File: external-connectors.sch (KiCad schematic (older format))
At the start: 7 parts, among them J1 Barrel_Jack +5V, J2 Barrel_Jack +12V, J3 Conn_02x10_Odd_Even, J4 Conn_02x08_Odd_Even, J5 Conn_02x08_Odd_Even

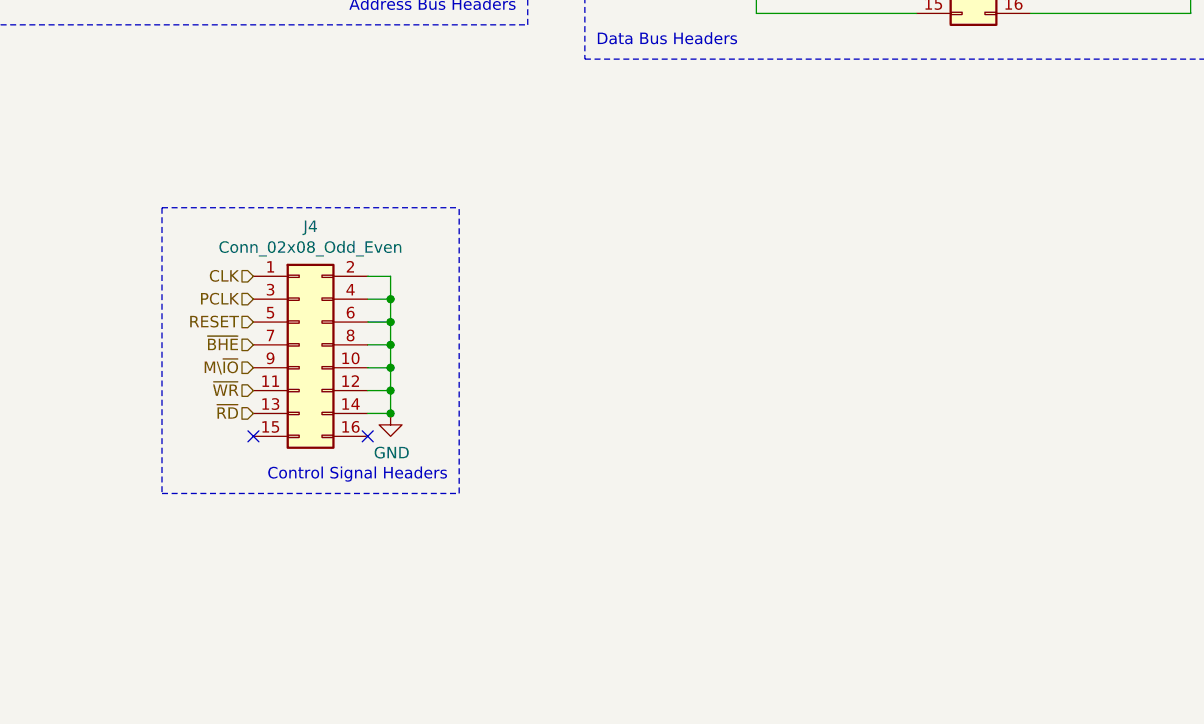
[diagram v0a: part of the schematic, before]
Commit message: assign footprints and edits
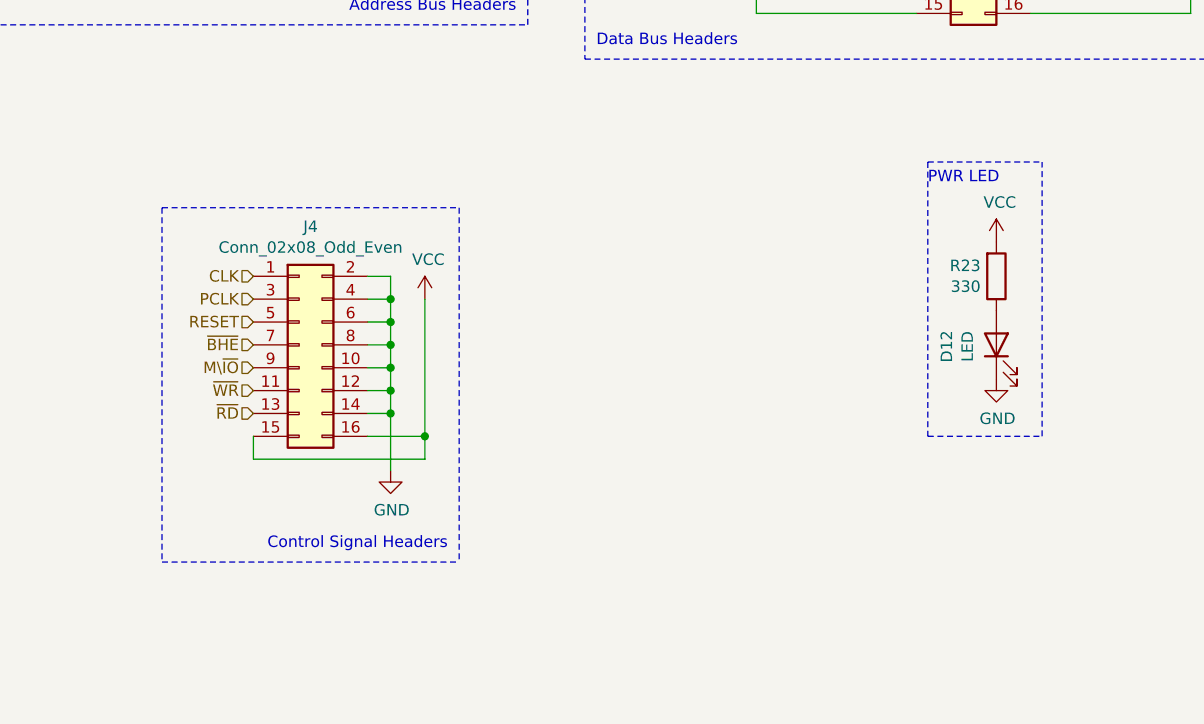
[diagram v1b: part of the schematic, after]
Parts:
- added D12: LED, LED_THT:LED_D5.0mm, symbol Device:LED
- added R23: 330, Resistor_THT:R_Axial_DIN0207_L6.3mm_D2.5mm_P10.16mm_Horizontal, symbol Device:R
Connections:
- net GND: now also D12.1 (K)
- net VCC: now also J4.15 (Pin_15), J4.16 (Pin_16), R23.2
- new net: D12.2 (A), R23.1
- no-connect marks 2 -> 0
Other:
- note added: "PWR LED"
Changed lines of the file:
@@
 $EndComp
 Wire Notes Line
-	3700 4450 3700 5700
-Wire Notes Line
-	3700 5700 5000 5700
-Wire Notes Line
-	5000 5700 5000 4450
+	3700 6000 5000 6000
 Wire Notes Line
 	3700 4450 5000 4450
-Text Notes 4950 5650 2    50   ~ 0
+Text Notes 4950 5950 2    50   ~ 0
 Control Signal Headers
 Text HLabel 4100 5150 0    50   Input ~ 0
@@
 Text HLabel 4100 5350 0    50   Input ~ 0
 ~RD
-NoConn ~ 4100 5450
-NoConn ~ 4600 5450
 Wire Wire Line
 	4600 4750 4700 4750
@@
 L power:GND #PWR0105
 U 1 1 62100CCC
-P 4700 5350
-F 0 "#PWR0105" H 4700 5100 50  0001 C CNN
-F 1 "GND" H 4705 5177 50  0000 C CNN
-F 2 "" H 4700 5350 50  0001 C CNN
-F 3 "" H 4700 5350 50  0001 C CNN
-	1    4700 5350
+P 4700 5600
+F 0 "#PWR0105" H 4700 5350 50  0001 C CNN
+F 1 "GND" H 4705 5427 50  0000 C CNN
+F 2 "" H 4700 5600 50  0001 C CNN
+F 3 "" H 4700 5600 50  0001 C CNN
+	1    4700 5600
 	1    0    0    -1
 $EndComp
@@
 	4700 5250 4700 5350
 Connection ~ 4700 5250
-Connection ~ 4700 5350
 $Comp
 L power:PWR_FLAG #FLG0101
@@
 	2450 5500 1850 5500
 Connection ~ 1850 5500
+Text Notes 7050 4350 0    50   ~ 0
+PWR LED
+$Comp
+L power:VCC #PWR02
+U 1 1 61BA534A
+P 7350 4600
+F 0 "#PWR02" H 7350 4450 50  0001 C CNN
+F 1 "VCC" H 7365 4773 50  0000 C CNN
+F 2 "" H 7350 4600 50  0001 C CNN
+F 3 "" H 7350 4600 50  0001 C CNN
+	1    7350 4600
+	1    0    0    -1
+$EndComp
+$Comp
+L power:GND #PWR03
+U 1 1 61BA5A77
+P 7350 5200
+F 0 "#PWR03" H 7350 4950 50  0001 C CNN
+F 1 "GND" H 7355 5027 50  0000 C CNN
+F 2 "" H 7350 5200 50  0001 C CNN
+F 3 "" H 7350 5200 50  0001 C CNN
+	1    7350 5200
+	1    0    0    -1
+$EndComp
+Wire Wire Line
+	4100 5450 4100 5550
+Wire Wire Line
+	4100 5550 4850 5550
+Wire Wire Line
+	4850 5550 4850 5450
+Wire Wire Line
+	4700 5600 4700 5350
+Connection ~ 4700 5350
+$Comp
+L power:VCC #PWR01
+U 1 1 61BBFA03
+P 4850 4850
+F 0 "#PWR01" H 4850 4700 50  0001 C CNN
+F 1 "VCC" H 4865 5023 50  0000 C CNN
+F 2 "" H 4850 4850 50  0001 C CNN
+F 3 "" H 4850 4850 50  0001 C CNN
+	1    4850 4850
+	1    0    0    -1
+$EndComp
+Wire Wire Line
+	4600 5450 4850 5450
+Connection ~ 4850 5450
+Wire Wire Line
+	4850 5450 4850 4850
+Wire Notes Line
+	5000 4450 5000 6000
+Wire Notes Line
+	3700 4450 3700 6000
+$Comp
+L Device:LED D?
+U 1 1 61BD0CAA
+P 7350 5050
+AR Path="/61CCC9EF/61BD0CAA" Ref="D?"  Part="1"
+AR Path="/626E3AF4/61BD0CAA" Ref="D12"  Part="1"
+F 0 "D12" H 7343 5267 50  0000 C CNN
+F 1 "LED" H 7343 5176 50  0000 C CNN
+F 2 "LED_THT:LED_D5.0mm" H 7350 5050 50  0001 C CNN
+F 3 "~" H 7350 5050 50  0001 C CNN
+	1    7350 5050
+	0    -1   -1   0
+$EndComp
+$Comp
+L Device:R R23
+U 1 1 61BD3D88
+P 7350 4750
+F 0 "R23" H 7281 4704 50  0000 R CNN
+F 1 "330" H 7281 4795 50  0000 R CNN
+F 2 "Resistor_THT:R_Axial_DIN0207_L6.3mm_D2.5mm_P10.16mm_Horizontal" V 7280 4750 50  0001 C CNN
+F 3 "~" H 7350 4750 50  0001 C CNN
+	1    7350 4750
+	1    0    0    1
+$EndComp
+Wire Notes Line
+	7050 4250 7050 5450
+Wire Notes Line
+	7050 5450 7550 5450
+Wire Notes Line
+	7550 5450 7550 4250
+Wire Notes Line
+	7050 4250 7550 4250
 Wire Bus Line
 	6050 1950 8100 1950
